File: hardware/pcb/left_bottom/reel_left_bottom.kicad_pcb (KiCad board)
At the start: 2 copper layers, 145.9 x 95.9 mm, 5 parts

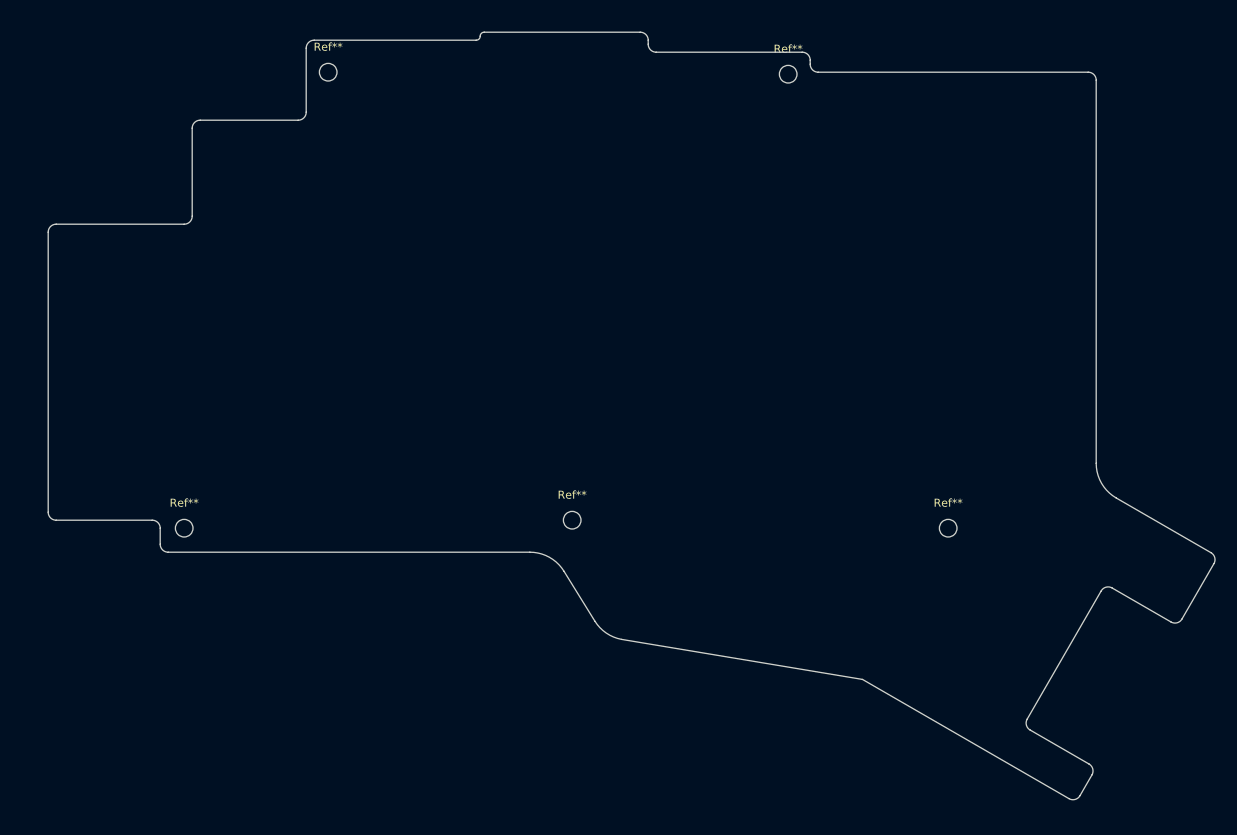
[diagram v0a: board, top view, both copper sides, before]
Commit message: Publish current hardware and fabrication assets
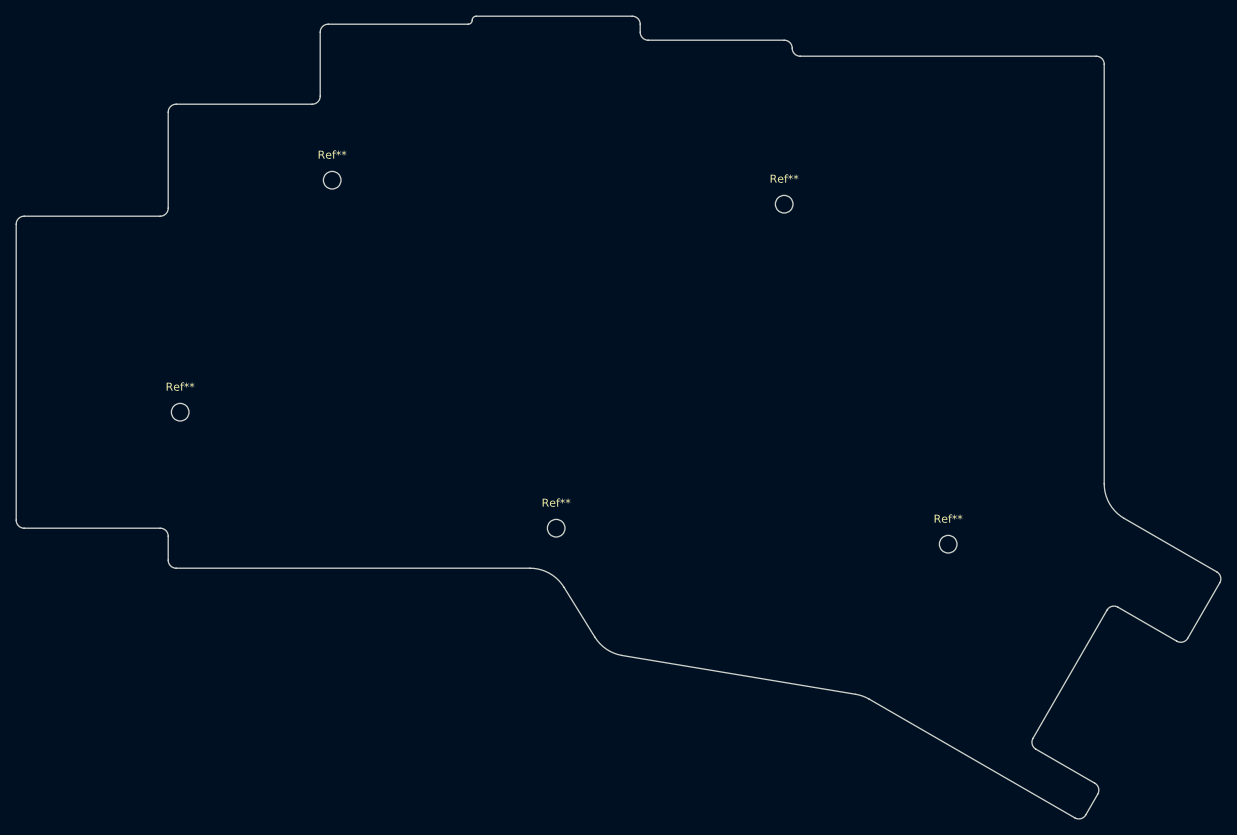
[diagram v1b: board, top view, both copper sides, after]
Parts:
- removed the Ref** at (169.5, 58.2)
- removed the Ref** at (142.5, 114.0)
- removed the Ref** at (189.5, 115.0)
- removed the Ref** at (94.0, 115.0)
- removed the Ref** at (112.0, 58.0)
- added Ref**: MountingHole_2.2mm_M2, MountingHole:MountingHole_2.2mm_M2, F.Cu at (93.5, 100.5)
- added Ref**: MountingHole_2.2mm_M2, MountingHole:MountingHole_2.2mm_M2, F.Cu at (112.5, 71.5)
- added Ref**: MountingHole_2.2mm_M2, MountingHole:MountingHole_2.2mm_M2, F.Cu at (189.5, 117.0)
- added Ref**: MountingHole_2.2mm_M2, MountingHole:MountingHole_2.2mm_M2, F.Cu at (140.5, 115.0)
- added Ref**: MountingHole_2.2mm_M2, MountingHole:MountingHole_2.2mm_M2, F.Cu at (169.0, 74.5)
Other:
- board size 145.9 x 95.9 mm -> 150.6 x 100.3 mm
